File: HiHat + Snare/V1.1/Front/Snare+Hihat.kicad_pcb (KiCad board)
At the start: 2 copper layers, 40 x 128 mm, 4 parts

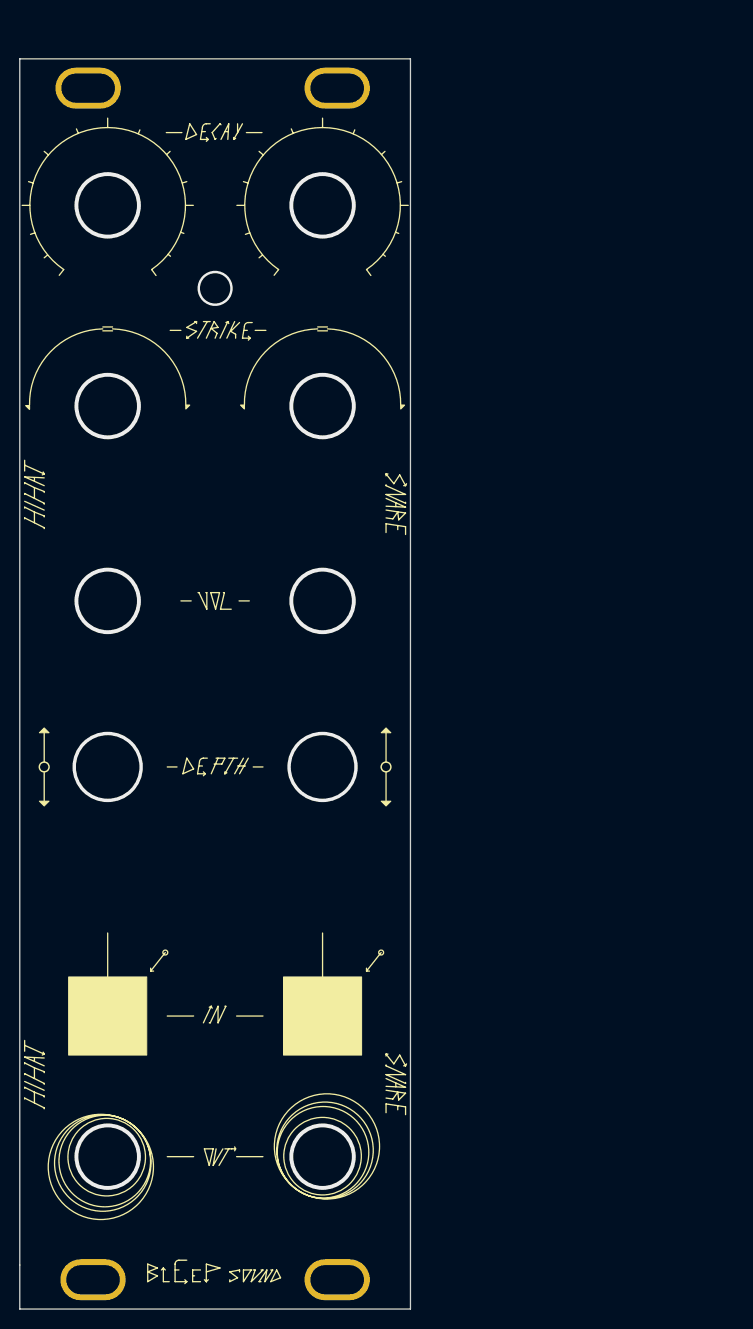
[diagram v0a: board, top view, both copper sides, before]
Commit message: add gerber files
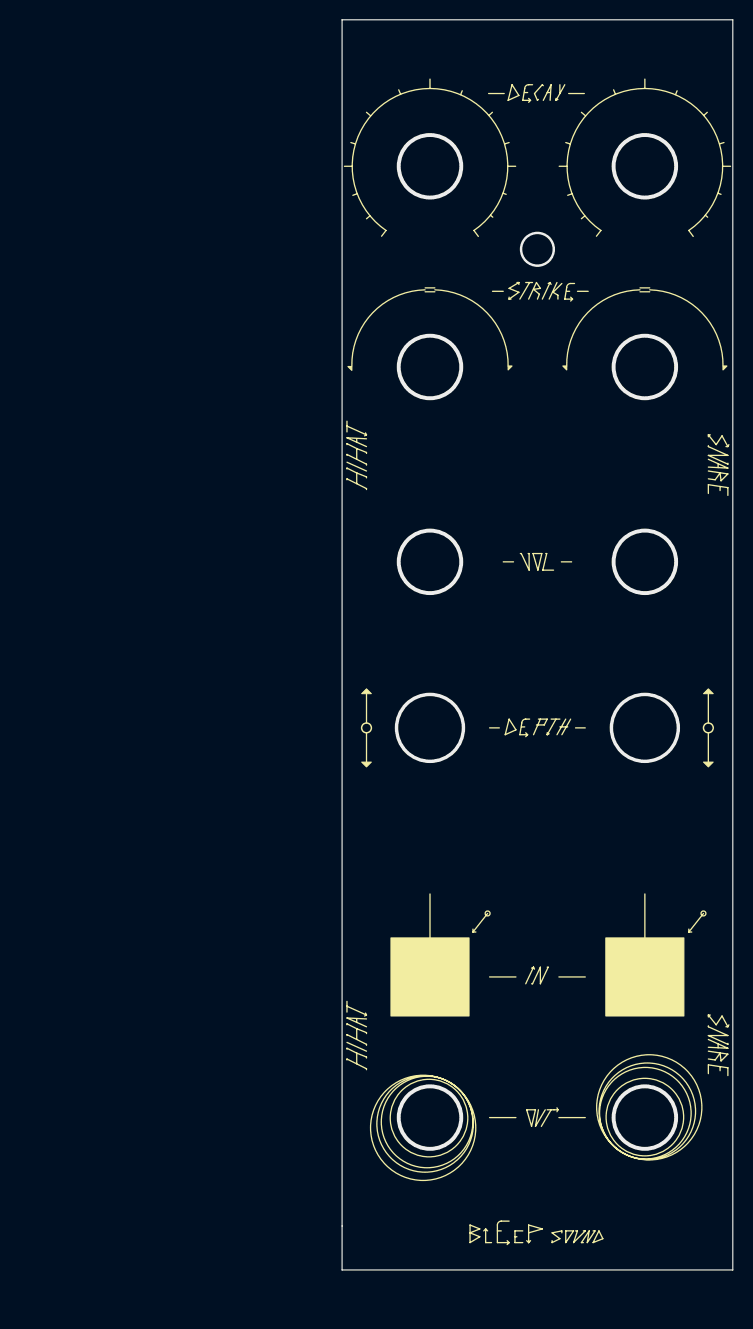
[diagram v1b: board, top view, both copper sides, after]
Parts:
- removed REF** (x4): Doepfer Mounting hole, Synth:Doepfer Mounting hole
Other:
- board text added: "Front panel"
- board text added: "Snare + HiHat V1.1 BleepSound 2022"
